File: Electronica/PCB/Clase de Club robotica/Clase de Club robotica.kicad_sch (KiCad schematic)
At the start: 17 parts, among them J1 Ultrasonico 1, J2 Screw_Terminal_01x02, J3 Ultrasonico 2, J4 Ultrasonico 3, J6 Screw_Terminal_01x02, SW1 SW_SPST, SW2 SW_Push

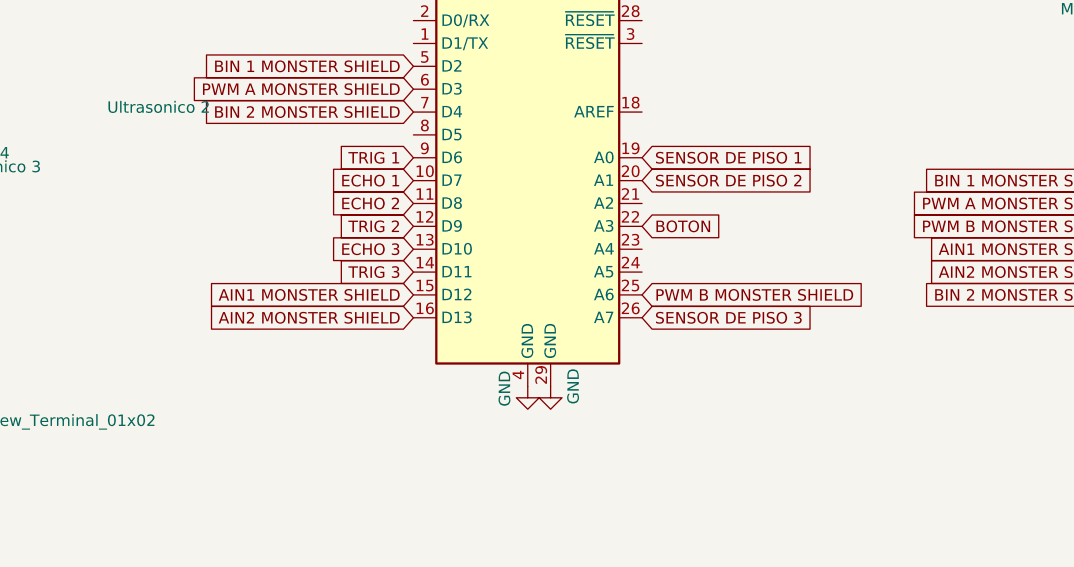
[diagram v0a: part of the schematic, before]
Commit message: 4 puentes
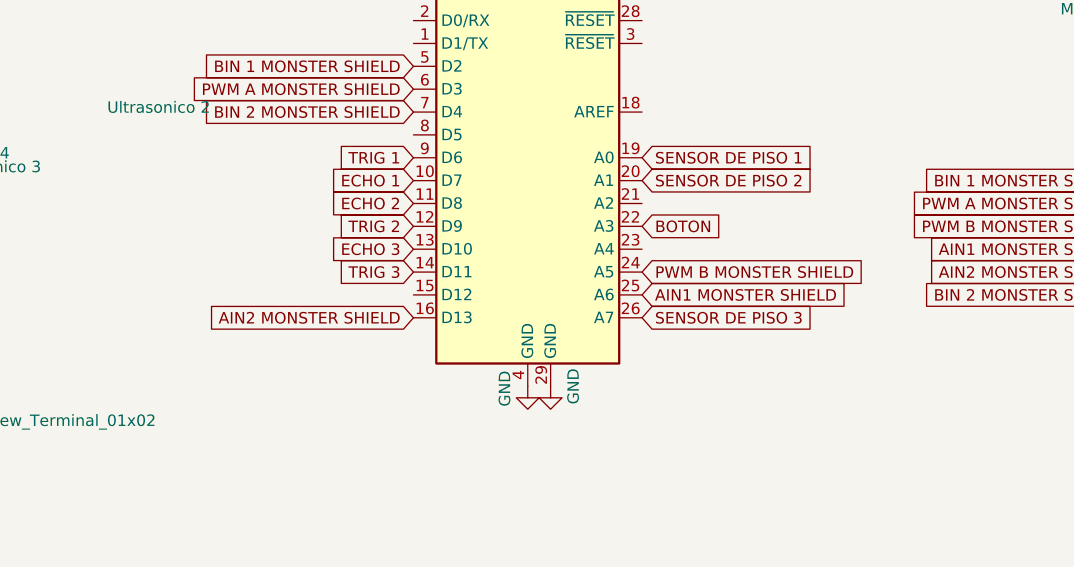
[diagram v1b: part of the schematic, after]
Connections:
- net AIN1 MONSTER SHIELD: now also A1.25 (A6); no longer A1.15 (D12)
- net PWM B MONSTER SHIELD: now also A1.24 (A5); no longer A1.25 (A6)
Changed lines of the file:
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@@
 	(global_label "AIN1 MONSTER SHIELD"
 		(shape input)
-		(at 158.75 73.66 180)
-		(fields_autoplaced yes)
-		(effects
-			(font
-				(size 1.27 1.27)
-			)
-			(justify right)
-		)
-		(property "Intersheetrefs" "${INTERSHEET_REFS}"
-			(at 134.2958 73.66 0)
-			(effects
-				(font
-					(size 1.27 1.27)
-				)
-				(justify right)
+		(at 184.15 73.66 0)
+		(fields_autoplaced yes)
+		(effects
+			(font
+				(size 1.27 1.27)
+			)
+			(justify left)
+		)
+		(property "Intersheetrefs" "${INTERSHEET_REFS}"
+			(at 208.6042 73.66 0)
+			(effects
+				(font
+					(size 1.27 1.27)
+				)
+				(justify left)
 				(hide yes)
 			)
@@
 	(global_label "PWM B MONSTER SHIELD"
 		(shape input)
-		(at 184.15 73.66 0)
+		(at 184.15 71.12 0)
 		(fields_autoplaced yes)
 		(effects
@@
 		)
 		(property "Intersheetrefs" "${INTERSHEET_REFS}"
-			(at 210.7812 73.66 0)
-			(effects
-				(font
+			(at 210.7812 71.12 0)
+			(effects
+				(font
